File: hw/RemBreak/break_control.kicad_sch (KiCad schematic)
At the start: 16 parts, among them J13 Conn_01x04, J4 Conn_01x07, J5 Conn_01x04, J6 Conn_01x01, J7 Conn_01x01, J8 Conn_01x07, J9 Conn_01x07, Q1 BC337, Q2 BC847

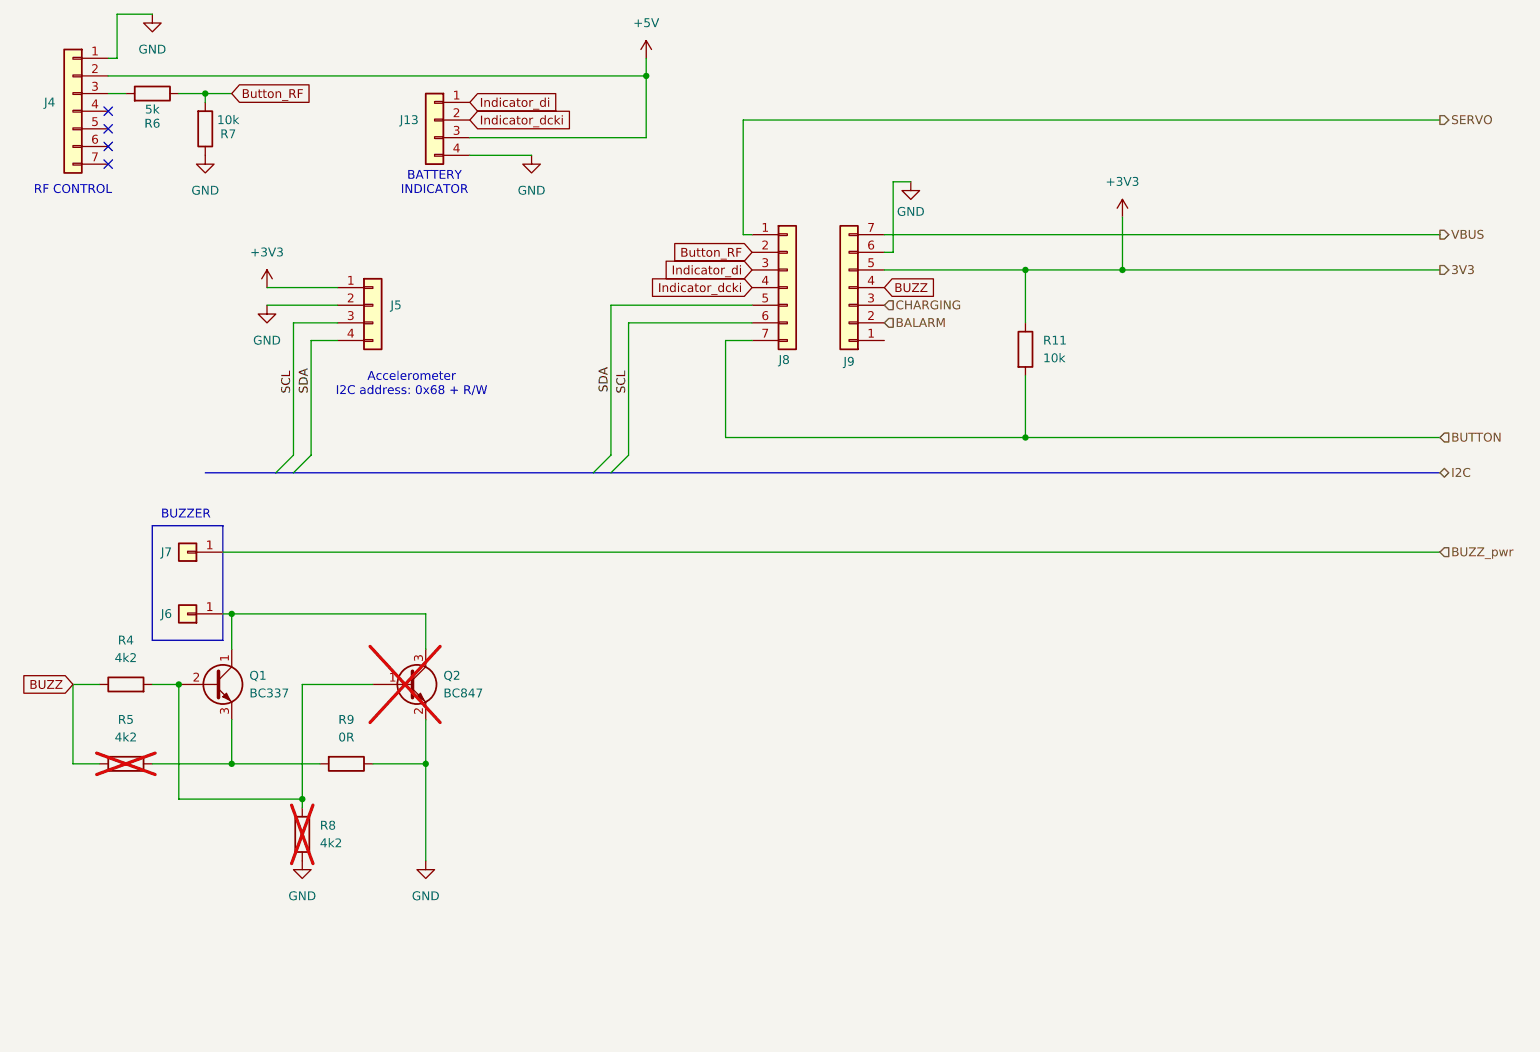
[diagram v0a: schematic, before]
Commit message: schematics development in progress
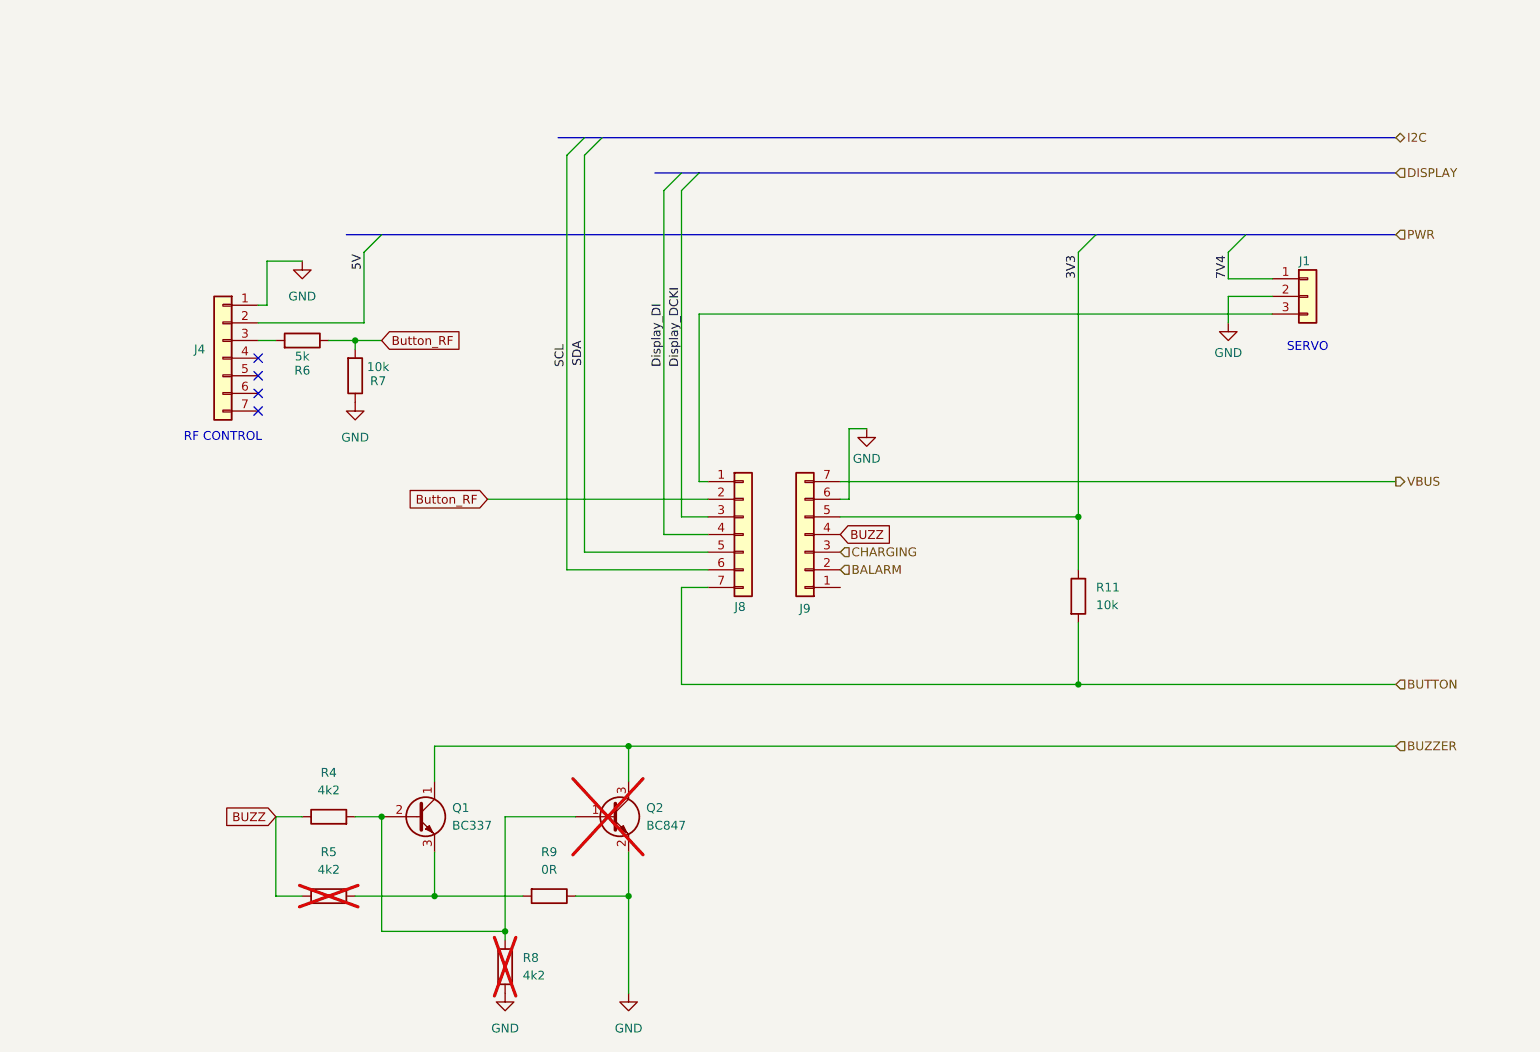
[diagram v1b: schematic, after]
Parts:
- removed J13, J5: Conn_01x04, Connector_PinSocket_2.54mm:PinSocket_1x04_P2.54mm_Vertical, symbol Connector_Generic:Conn_01x04
- removed J6, J7: Conn_01x01, TestPoint:TestPoint_Pad_2.5x2.5mm, symbol Connector_Generic:Conn_01x01
- added J1: Conn_01x03, Connector_PinHeader_2.54mm:PinHeader_1x03_P2.54mm_Vertical_SMD_Pin1Left, symbol Connector_Generic:Conn_01x03
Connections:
- net GND: now also J1.2 (Pin_2)
- net BUZZER: now reaches Q1.1 (C), Q2.3 (C)
- net +3V3 renamed 3V3
- net +5V renamed 5V
- net Indicator_dcki renamed Display_DI
- net Indicator_di renamed Display_DCKI
- net SERVO: no longer names the net of J8.1 (Pin_1)
- net SERVO: now also J1.3 (Pin_3)
- new net 7V4: J1.1 (Pin_1)
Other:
- note added: "SERVO"
- note removed: "Accelerometer I2C address: 0x68 + R/W"
- note removed: "BATTERY INDICATOR"
- note removed: "BUZZER"
- moved on the sheet: J4, J8, J9, Q1, Q2, R11, R4, R5, R6, R7, R8, R9

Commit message: updated pcb and schematics - still in progress
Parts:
- J4, J8, J9: footprint Connector_PinSocket_2.54mm:PinSocket_1x07_P2.54mm_Vertical -> Connector_PinSocket_2.54mm:PinSocket_1x07_P2.54mm_Vertical_SMD_Pin1Left
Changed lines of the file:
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@@
 			)
 		)
-		(property "Footprint" "Connector_PinSocket_2.54mm:PinSocket_1x07_P2.54mm_Vertical"
+		(property "Footprint" "Connector_PinSocket_2.54mm:PinSocket_1x07_P2.54mm_Vertical_SMD_Pin1Left"
 			(at 143.51 93.98 0)
 			(effects
@@
 			)
 		)
-		(property "Footprint" "Connector_PinSocket_2.54mm:PinSocket_1x07_P2.54mm_Vertical"
+		(property "Footprint" "Connector_PinSocket_2.54mm:PinSocket_1x07_P2.54mm_Vertical_SMD_Pin1Left"
 			(at 59.69 68.58 0)
 			(effects
@@
 			)
 		)
-		(property "Footprint" "Connector_PinSocket_2.54mm:PinSocket_1x07_P2.54mm_Vertical"
+		(property "Footprint" "Connector_PinSocket_2.54mm:PinSocket_1x07_P2.54mm_Vertical_SMD_Pin1Left"
 			(at 134.62 93.98 0)
 			(effects
